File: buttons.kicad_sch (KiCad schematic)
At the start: 96 parts, among them SW10 SW_MEC_5G, SW11 SW_MEC_5G, SW12 SW_MEC_5G, SW13 SW_MEC_5G, SW14 SW_MEC_5G, SW15 SW_MEC_5G, SW16 SW_MEC_5G, SW17 SW_MEC_5G, SW18 SW_MEC_5G, SW19 SW_MEC_5G, SW2 SW_MEC_5G, SW20 SW_MEC_5G, SW21 SW_MEC_5G, SW22 SW_MEC_5G, SW23 SW_MEC_5G, SW24 SW_MEC_5G, SW25 SW_MEC_5G, SW26 SW_MEC_5G, SW27 SW_MEC_5G, SW28 SW_MEC_5G, SW29 SW_MEC_5G, SW3 SW_MEC_5G, SW30 SW_MEC_5G, SW31 SW_MEC_5G, SW32 SW_MEC_5G, SW33 SW_MEC_5G, SW34 SW_MEC_5G, SW35 SW_MEC_5G, SW36 SW_MEC_5G, SW37 SW_MEC_5G, SW38 SW_MEC_5G, SW39 SW_MEC_5G, SW4 SW_MEC_5G, SW40 SW_MEC_5G, SW41 SW_MEC_5G, SW42 SW_MEC_5G, SW43 SW_MEC_5G, SW44 SW_MEC_5G, SW45 SW_MEC_5G, SW46 SW_MEC_5G, SW47 SW_MEC_5G, SW48 SW_MEC_5G, SW49 SW_MEC_5G, SW5 SW_MEC_5G, SW6 SW_MEC_5G, SW7 SW_MEC_5G, SW8 SW_MEC_5G, SW9 SW_MEC_5G

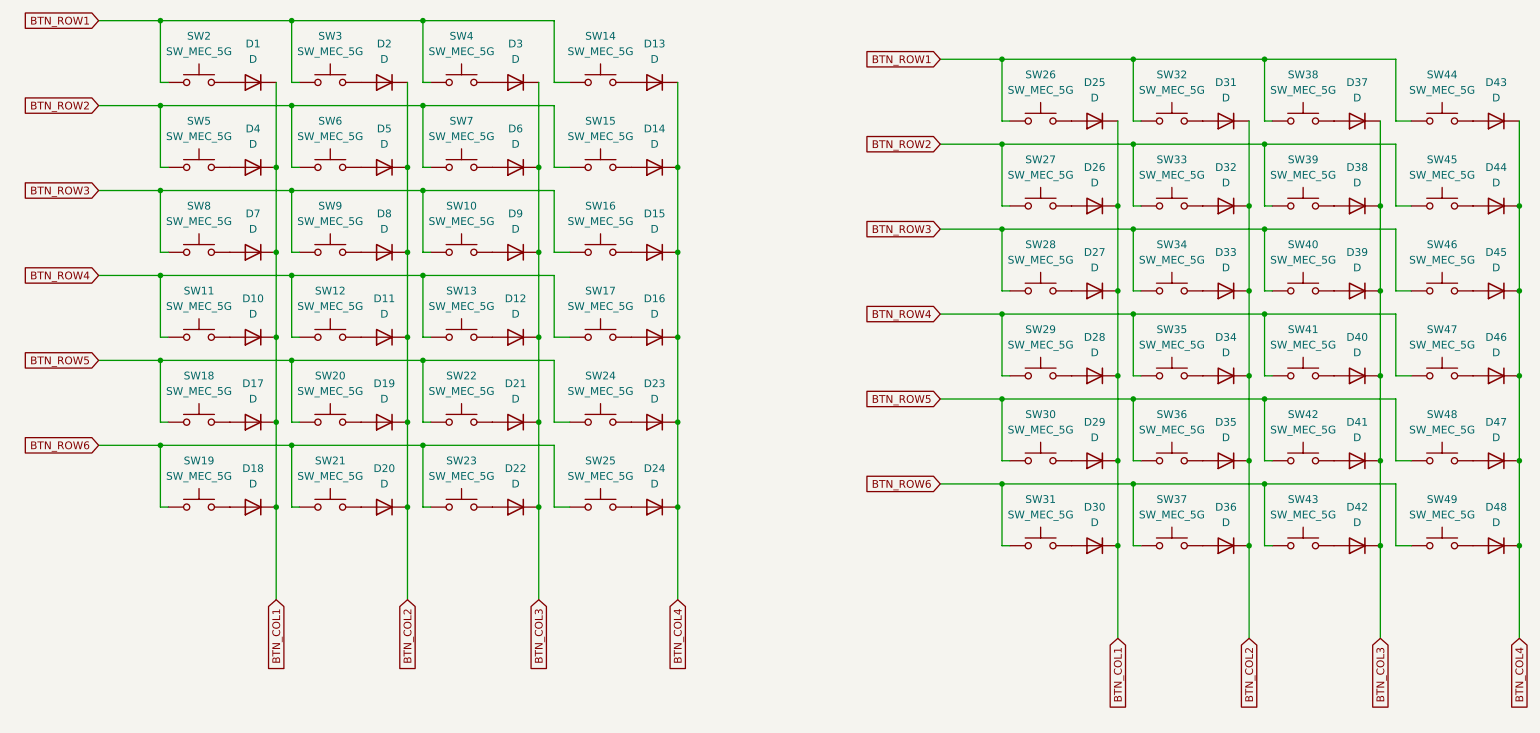
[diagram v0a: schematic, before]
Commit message: pcb
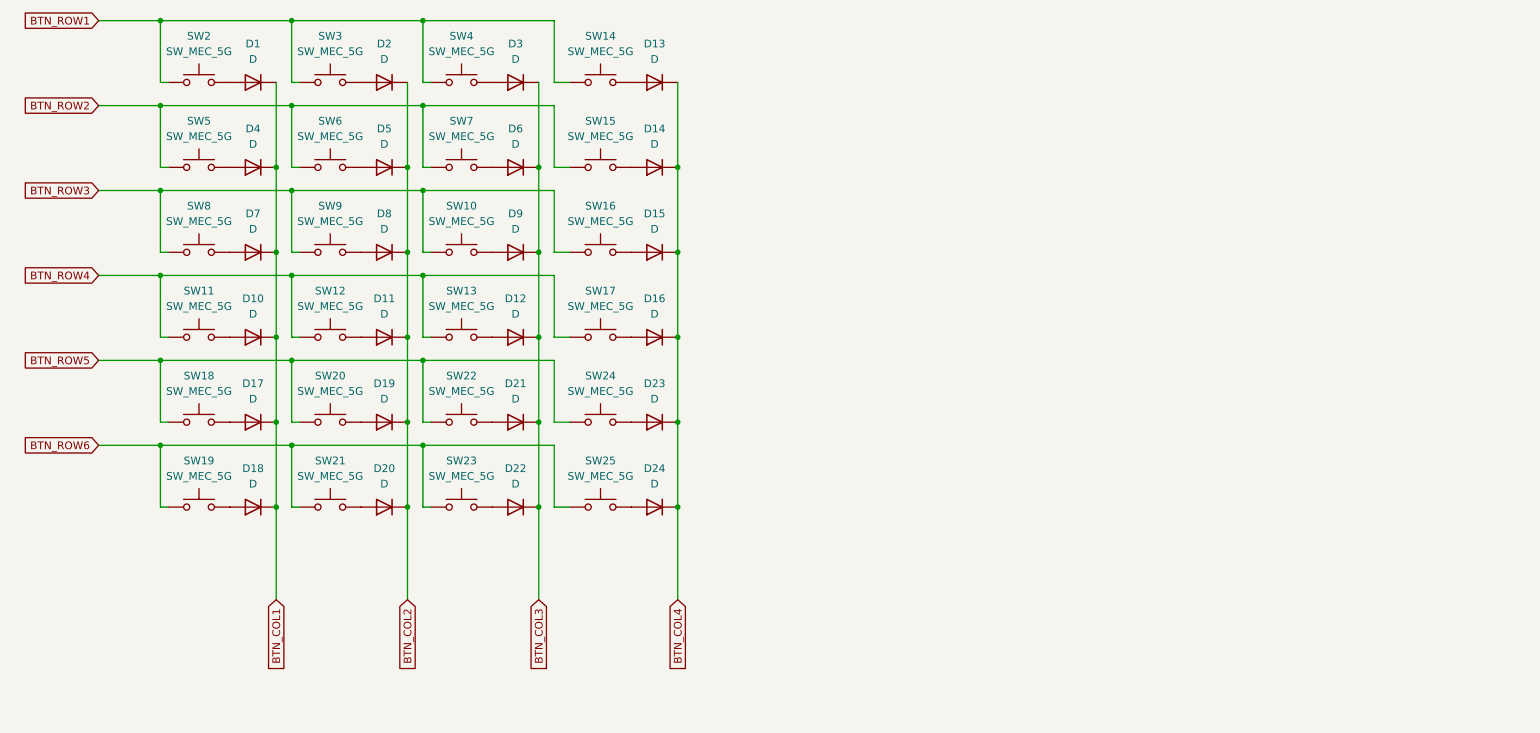
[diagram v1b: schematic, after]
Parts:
- removed D25, D26, D27, D28, D29, D30, D31, D32, D33, D34, D35, D36, D37, D38, D39, D40, D41, D42, D43, D44, D45, D46, D47, D48: D, symbol Device:D
- removed SW26, SW27, SW28, SW29, SW30, SW31, SW32, SW33, SW34, SW35, SW36, SW37, SW38, SW39, SW40, SW41, SW42, SW43, SW44, SW45, SW46, SW47, SW48, SW49: SW_MEC_5G, symbol Switch:SW_MEC_5G
